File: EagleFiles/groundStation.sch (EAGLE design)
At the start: 5 parts

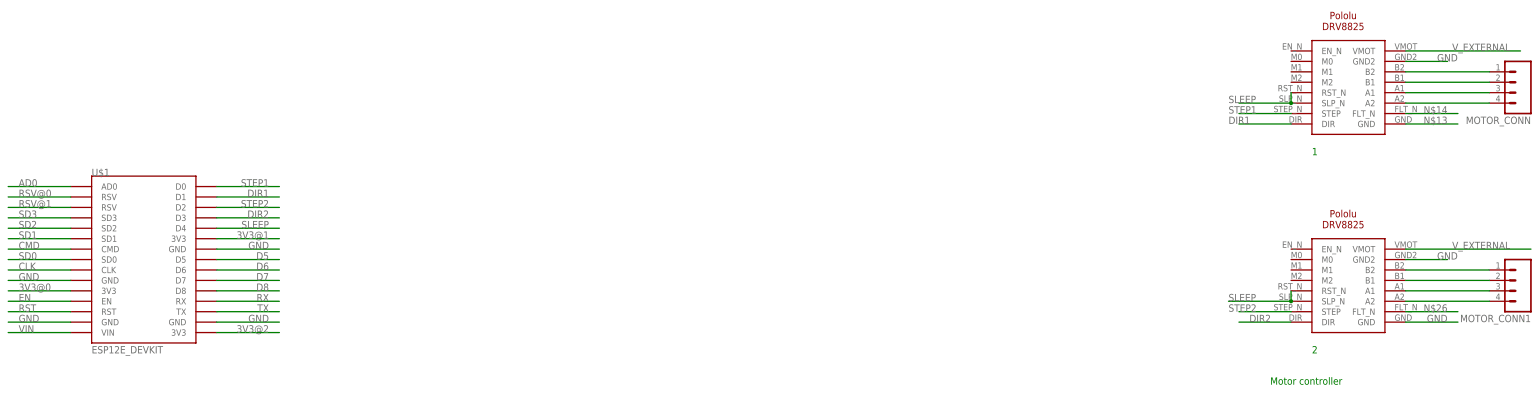
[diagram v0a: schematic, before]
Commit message: small changes in motor control
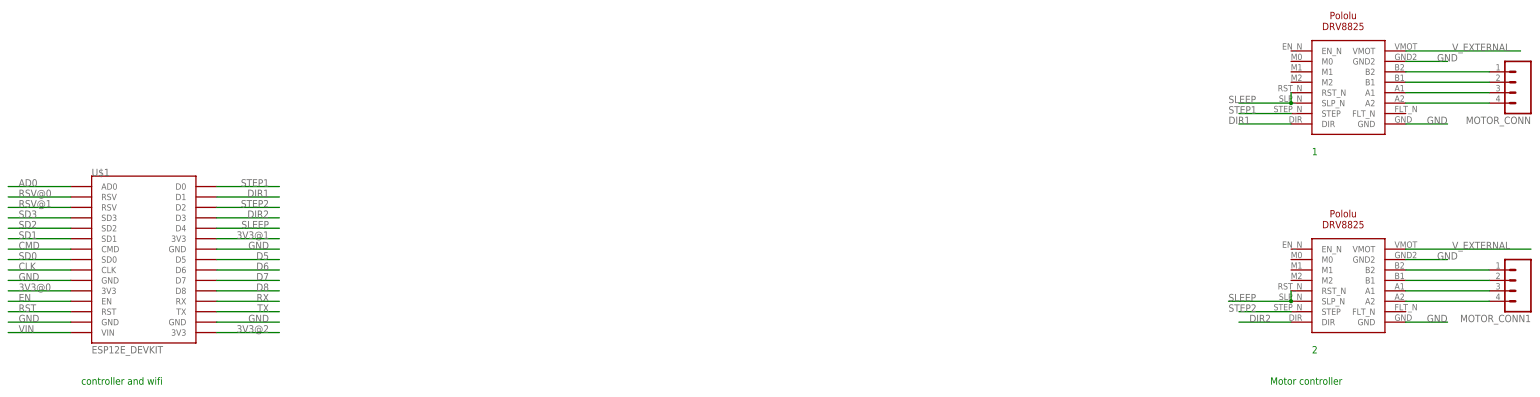
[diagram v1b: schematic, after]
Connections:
- removed net N$13: U$2.GND
- removed net N$14: U$2.FLT_N
- removed net N$26: U$4.FLT_N
- net GND: now also U$2.GND
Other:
- note added: "controller and wifi"
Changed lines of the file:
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@@
 <text x="302.26" y="78.74" size="1.778" layer="91">1</text>
 <text x="302.26" y="30.48" size="1.778" layer="91">2</text>
+<text x="2.54" y="22.86" size="1.778" layer="91">controller and wifi</text>
 </plain>
 <instances>
@@
 <segment>
 <pinref part="U$4" gate="G$1" pin="GND"/>
-<wire x1="325.12" y1="38.1" x2="337.82" y2="38.1" width="0.1524" layer="91"/>
+<wire x1="325.12" y1="38.1" x2="335.28" y2="38.1" width="0.1524" layer="91"/>
 <label x="335.28" y="38.1" size="1.778" layer="95" align="bottom-right"/>
 </segment>
@@
 <wire x1="0" y1="38.1" x2="-15.24" y2="38.1" width="0.1524" layer="91"/>
 <label x="-12.7" y="38.1" size="1.778" layer="95"/>
+</segment>
+<segment>
+<pinref part="U$2" gate="G$1" pin="GND"/>
+<wire x1="325.12" y1="86.36" x2="335.28" y2="86.36" width="0.1524" layer="91"/>
+<label x="335.28" y="86.36" size="1.778" layer="95" align="bottom-right"/>
 </segment>
 </net>
@@
 </segment>
 </net>
-<net name="N$13" class="0">
-<segment>
-<pinref part="U$2" gate="G$1" pin="GND"/>
-<wire x1="325.12" y1="86.36" x2="337.82" y2="86.36" width="0.1524" layer="91"/>
-<label x="335.28" y="86.36" size="1.778" layer="95" align="bottom-right"/>
-</segment>
-</net>
-<net name="N$14" class="0">
-<segment>
-<pinref part="U$2" gate="G$1" pin="FLT_N"/>
-<wire x1="325.12" y1="88.9" x2="337.82" y2="88.9" width="0.1524" layer="91"/>
-<label x="335.28" y="88.9" size="1.778" layer="95" align="bottom-right"/>
-</segment>
-</net>
 <net name="V_EXTERNAL" class="0">
 <segment>
@@
 </segment>
 </net>
-<net name="N$26" class="0">
-<segment>
-<pinref part="U$4" gate="G$1" pin="FLT_N"/>
-<wire x1="325.12" y1="40.64" x2="337.82" y2="40.64" width="0.1524" layer="91"/>
-<label x="335.28" y="40.64" size="1.778" layer="95" align="bottom-right"/>
-</segment>
-</net>
